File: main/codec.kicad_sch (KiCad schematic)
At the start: 17 parts, among them J1 AudioJack5, U2 TLV320AIC3104IRHBR, U200 AP2120N-1.8TRG1

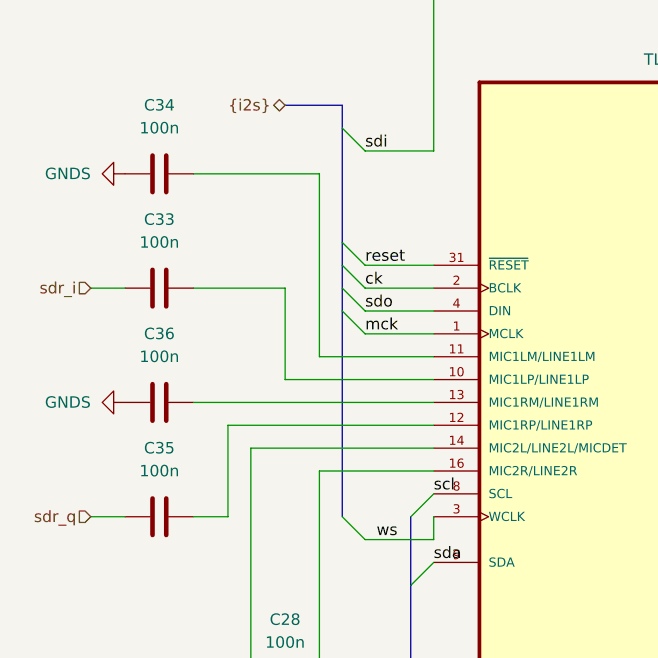
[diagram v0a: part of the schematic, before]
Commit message: mixer connected, MCU wiring changed
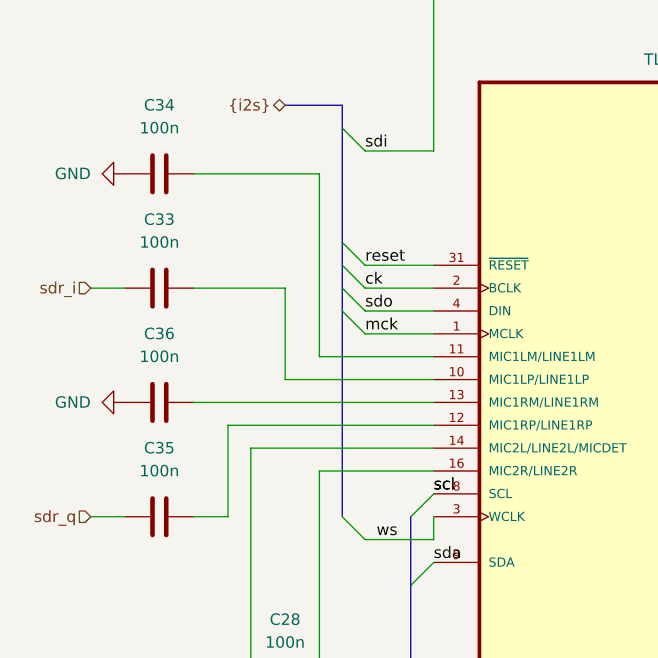
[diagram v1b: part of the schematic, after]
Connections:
- net GNDS is gone; now on net GND: C34.1, C36.1
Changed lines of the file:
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@@
+    (stroke (width 0) (type default))
+  )
+  (bus_entry (at 81.28 93.98) (size 2.54 2.54)
+    (stroke (width 0) (type default))
+  )
+  (bus_entry (at 81.28 96.52) (size 2.54 2.54)
+    (stroke (width 0) (type default))
+  )
+  (bus_entry (at 81.28 91.44) (size 2.54 2.54)
     (stroke (width 0) (type default))
   )
   (bus_entry (at 88.9 119.38) (size 2.54 -2.54)
-    (stroke (width 0) (type default))
-  )
-  (bus_entry (at 81.28 93.98) (size 2.54 2.54)
-    (stroke (width 0) (type default))
-  )
-  (bus_entry (at 81.28 96.52) (size 2.54 2.54)
-    (stroke (width 0) (type default))
-  )
-  (bus_entry (at 81.28 91.44) (size 2.54 2.54)
     (stroke (width 0) (type default))
   )
@@
     (effects (font (size 1.27 1.27)) (justify left bottom))
   )
+  (label "scl" (at 91.44 116.84 0)
+    (effects (font (size 1.27 1.27)) (justify left bottom))
+  )
   (label "reset" (at 83.82 91.44 0) (fields_autoplaced)
     (effects (font (size 1.27 1.27)) (justify left bottom))
@@
   (hierarchical_label "VOUTR-" (shape output) (at 157.48 111.76 0) (fields_autoplaced)
     (effects (font (size 1.27 1.27)) (justify left))
+  )
+  (symbol (lib_id "power:GND") (at 57.15 81.28 270) (unit 1)
+    (in_bom yes) (on_board yes) (dnp no) (fields_autoplaced)
+    (property "Reference" "#PWR018" (at 50.8 81.28 0)
+      (effects (font (size 1.27 1.27)) hide)
+    )
+    (property "Value" "GND" (at 53.34 81.28 90)
+      (effects (font (size 1.27 1.27)) (justify right))
+    )
+    (property "Footprint" "" (at 57.15 81.28 0)
+      (effects (font (size 1.27 1.27)) hide)
+    )
+    (property "Datasheet" "" (at 57.15 81.28 0)
+      (effects (font (size 1.27 1.27)) hide)
+    )
+    (pin "1")
+    (instances
+      (project "main"
+        (path "/cb08c644-d155-44e5-86e1-31645eace055/e511764a-2dd7-4601-8d00-331d6dbffa9f"
+          (reference "#PWR018") (unit 1)
+        )
+      )
+    )
   )
   (symbol (lib_id "Device:C") (at 186.69 82.55 90) (unit 1)
@@
     )
   )
-  (symbol (lib_id "power:GNDS") (at 57.15 106.68 270) (unit 1)
-    (in_bom yes) (on_board yes) (dnp no) (fields_autoplaced)
-    (property "Reference" "#PWR018" (at 50.8 106.68 0)
-      (effects (font (size 1.27 1.27)) hide)
-    )
-    (property "Value" "GNDS" (at 53.34 106.68 90)
-      (effects (font (size 1.27 1.27)) (justify right))
-    )
-    (property "Footprint" "" (at 57.15 106.68 0)
-      (effects (font (size 1.27 1.27)) hide)
-    )
-    (property "Datasheet" "" (at 57.15 106.68 0)
-      (effects (font (size 1.27 1.27)) hide)
-    )
-    (pin "1")
-    (instances
-      (project "main"
-        (path "/cb08c644-d155-44e5-86e1-31645eace055/e511764a-2dd7-4601-8d00-331d6dbffa9f"
-          (reference "#PWR018") (unit 1)
-        )
-      )
-    )
-  )
   (symbol (lib_id "power:GND") (at 109.22 41.91 0) (unit 1)
     (in_bom yes) (on_board yes) (dnp no) (fields_autoplaced)
@@
     )
   )
+  (symbol (lib_id "power:GND") (at 57.15 106.68 270) (unit 1)
+    (in_bom yes) (on_board yes) (dnp no) (fields_autoplaced)
+    (property "Reference" "#PWR020" (at 50.8 106.68 0)
+      (effects (font (size 1.27 1.27)) hide)
+    )
+    (property "Value" "GND" (at 53.34 106.68 90)
+      (effects (font (size 1.27 1.27)) (justify right))
+    )
+    (property "Footprint" "" (at 57.15 106.68 0)
+      (effects (font (size 1.27 1.27)) hide)
+    )
+    (property "Datasheet" "" (at 57.15 106.68 0)
+      (effects (font (size 1.27 1.27)) hide)
+    )
+    (pin "1")
+    (instances
+      (project "main"
+        (path "/cb08c644-d155-44e5-86e1-31645eace055/e511764a-2dd7-4601-8d00-331d6dbffa9f"
+          (reference "#PWR020") (unit 1)
+        )
+      )
+    )
+  )
   (symbol (lib_id "power:GND") (at 86.36 39.37 0) (unit 1)
     (in_bom yes) (on_board yes) (dnp no) (fields_autoplaced)
@@
         )
       )
-    )
-  )
-  (symbol (lib_id "power:GNDS") (at 57.15 81.28 270) (unit 1)
-    (in_bom yes) (on_board yes) (dnp no) (fields_autoplaced)
-    (property "Reference" "#PWR020" (at 50.8 81.28 0)
-      (effects (font (size 1.27 1.27)) hide)
-    )
-    (property "Value" "GNDS" (at 53.34 81.28 90)
-      (effects (font (size 1.27 1.27)) (justify right))
-    )
-    (property "Footprint" "" (at 57.15 81.28 0)
-      (effects (font (size 1.27 1.27)) hide)
-    )
-    (property "Datasheet" "" (at 57.15 81.28 0)
-      (effects (font (size 1.27 1.27)) hide)
-    )
-    (pin "1")
-    (instances
-      (project "main"
-        (path "/cb08c644-d155-44e5-86e1-31645eace055/e511764a-2dd7-4601-8d00-331d6dbffa9f"
-          (reference "#PWR020") (unit 1)
-        )
-      )

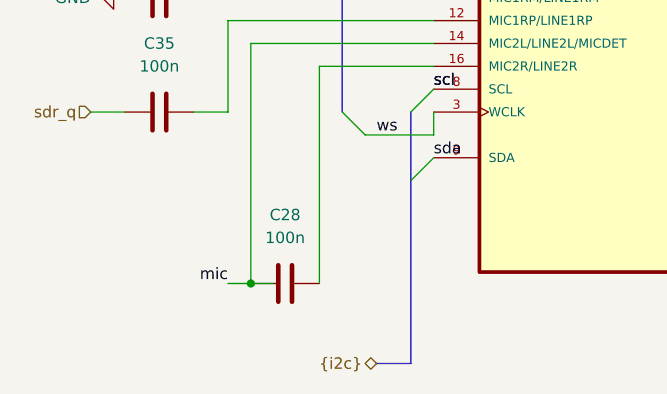
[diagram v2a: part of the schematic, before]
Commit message: Revire MCU to add swr_fwd and swr_rvs signals
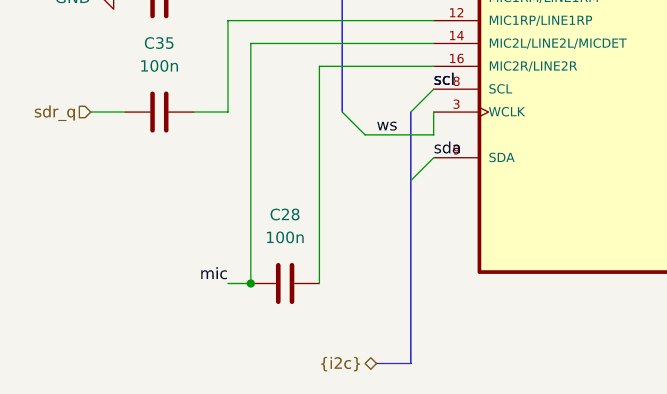
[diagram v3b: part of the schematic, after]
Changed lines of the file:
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@@
-    (stroke (width 0) (type default))
-  )
-  (wire (pts (xy 71.12 138.43) (xy 73.66 138.43))
     (stroke (width 0) (type default))
   )
